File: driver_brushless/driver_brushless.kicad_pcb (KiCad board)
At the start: 2 copper layers, 50 x 50 mm, 38 parts, among them U5 L6235D

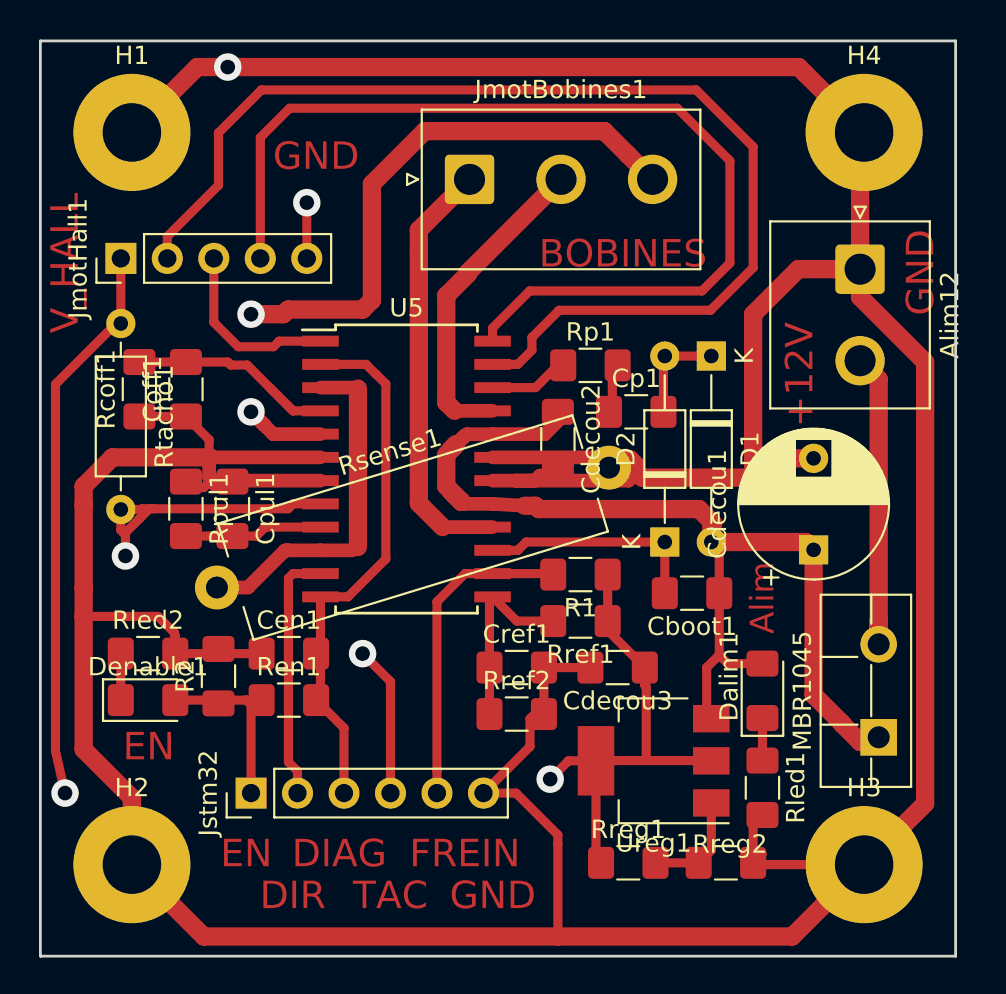
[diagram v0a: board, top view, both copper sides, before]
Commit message: afficheGrapheSerie
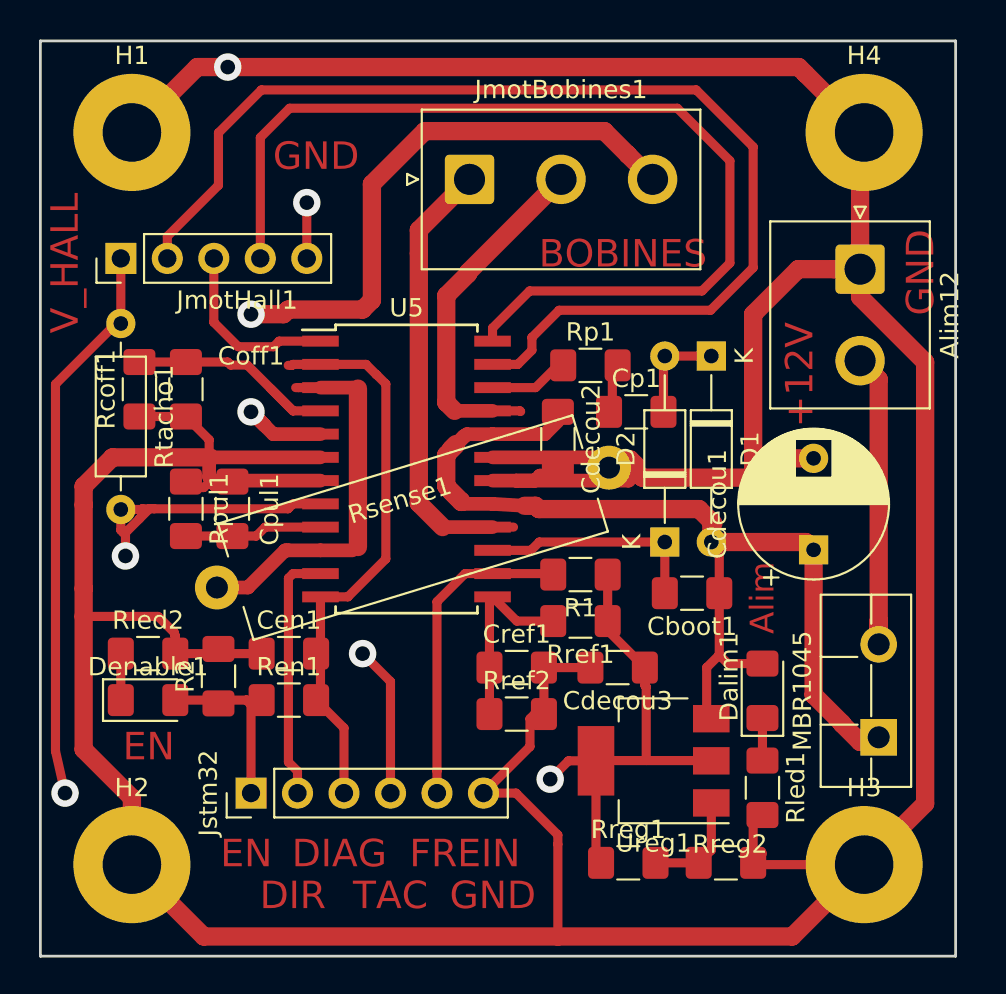
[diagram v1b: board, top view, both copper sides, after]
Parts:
- Ureg1: value LM317_3PinPackage -> LM317
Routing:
- net Net-(Cen1-Pad2): track 30.9 -> 32.6 mm
- net /Out_21: track 17.5 -> 19.1 mm
- net Net-(Rsense1-Pad1): track 20.1 -> 21.5 mm
- net /Out_31: track 23.4 -> 24.6 mm
